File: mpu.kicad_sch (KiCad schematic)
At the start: 1 part

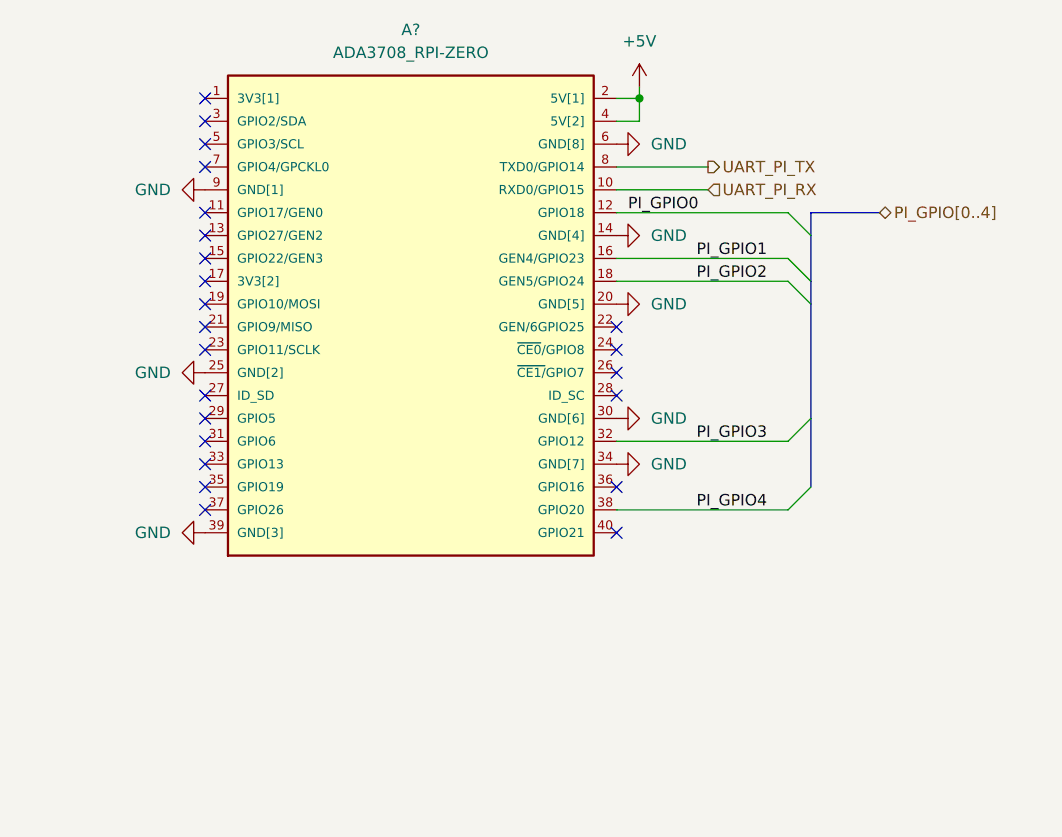
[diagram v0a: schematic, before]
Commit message: PCB Routing is done for first Proto
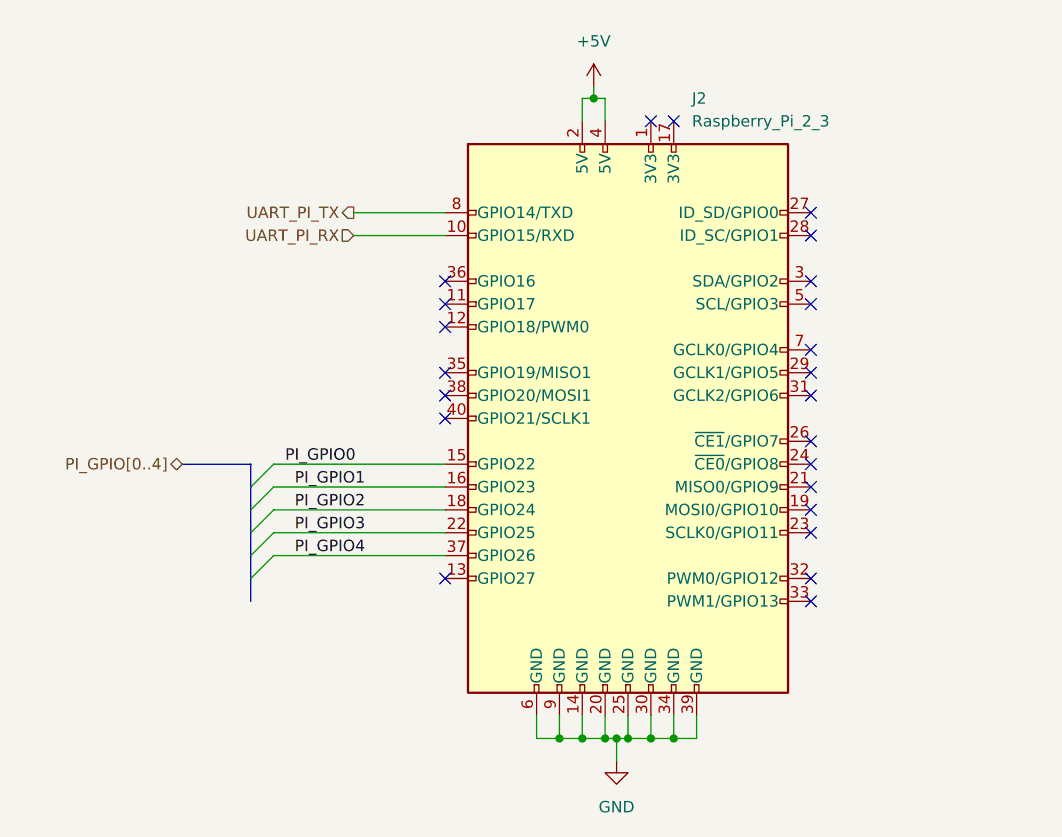
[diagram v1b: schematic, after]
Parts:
- removed A?: ADA3708_RPI-ZERO, SymLibs:ADA3708_RPI-ZERO, symbol ADA3708:ADA3708_RPI-ZERO
- added J2: Raspberry_Pi_2_3, Connector_PinSocket_2.54mm:PinSocket_2x20_P2.54mm_Vertical, symbol Connector:Raspberry_Pi_2_3
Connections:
- net +5V: now also J2.2 (5V), J2.4 (5V)
- net GND: now also J2.14 (GND), J2.20 (GND), J2.25 (GND), J2.30 (GND), J2.34 (GND), J2.39 (GND), J2.6 (GND), J2.9 (GND)
- net PI_GPIO0: now also J2.15 (GPIO22)
- net PI_GPIO1: now also J2.16 (GPIO23)
- net PI_GPIO2: now also J2.18 (GPIO24)
- net PI_GPIO3: now also J2.22 (GPIO25)
- net PI_GPIO4: now also J2.37 (GPIO26)
- net UART_PI_RX: now also J2.10 (GPIO15/RXD)
- net UART_PI_TX: now also J2.8 (GPIO14/TXD)
